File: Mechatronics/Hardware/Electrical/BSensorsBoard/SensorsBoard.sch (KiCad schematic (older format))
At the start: 5 parts, among them J1 Conn_01x01_Male, J2 Conn_01x01_Male, J3 Conn_01x01_Male, J4 Conn_01x01_Male, U1 ITR1802

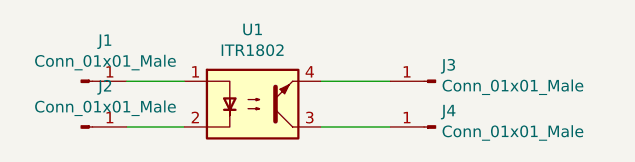
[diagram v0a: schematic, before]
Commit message: Changes
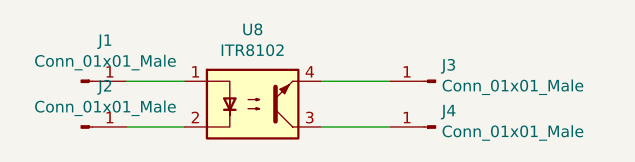
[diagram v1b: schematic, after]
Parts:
- U8: renamed from U1; value ITR1802 -> ITR8102
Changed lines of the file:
@@
 $EndDescr
 $Comp
-L SensorsBoard-rescue:ITR1802-Encoder U1
+L SensorsBoard-rescue:ITR1802-Encoder U8
 U 1 1 5C59CA18
 P 5900 4500
-F 0 "U1" H 5900 4825 50  0000 C CNN
-F 1 "ITR1802" H 5900 4734 50  0000 C CNN
+F 0 "U8" H 5900 4825 50  0000 C CNN
+F 1 "ITR8102" H 5900 4734 50  0000 C CNN
 F 2 "Encoder:itr8102" H 5900 4500 50  0001 C CNN
 F 3 "" H 5900 4500 50  0001 C CNN
